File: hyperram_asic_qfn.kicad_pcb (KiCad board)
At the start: 4 copper layers, 59.5 x 60 mm, 45 parts, among them IC1 W25Q32JVSSIQ_TR, IC2 S27KL0641DABHI020, IC3 LP5907UVX-1.8_NOPB, IC4 LP5907UVX-3.3_NOPB, IC5 LP5907MFX-3.3_NOPB, IC6 MCP1824T-1802E_OT, J1 USB_B_Micro, J2 Conn_02x03_Counter_Clockwise, J3 1156915, J4 1156915, U1 CARAVEL, Y1 SG5032CAN_20.000000M-TJGA3

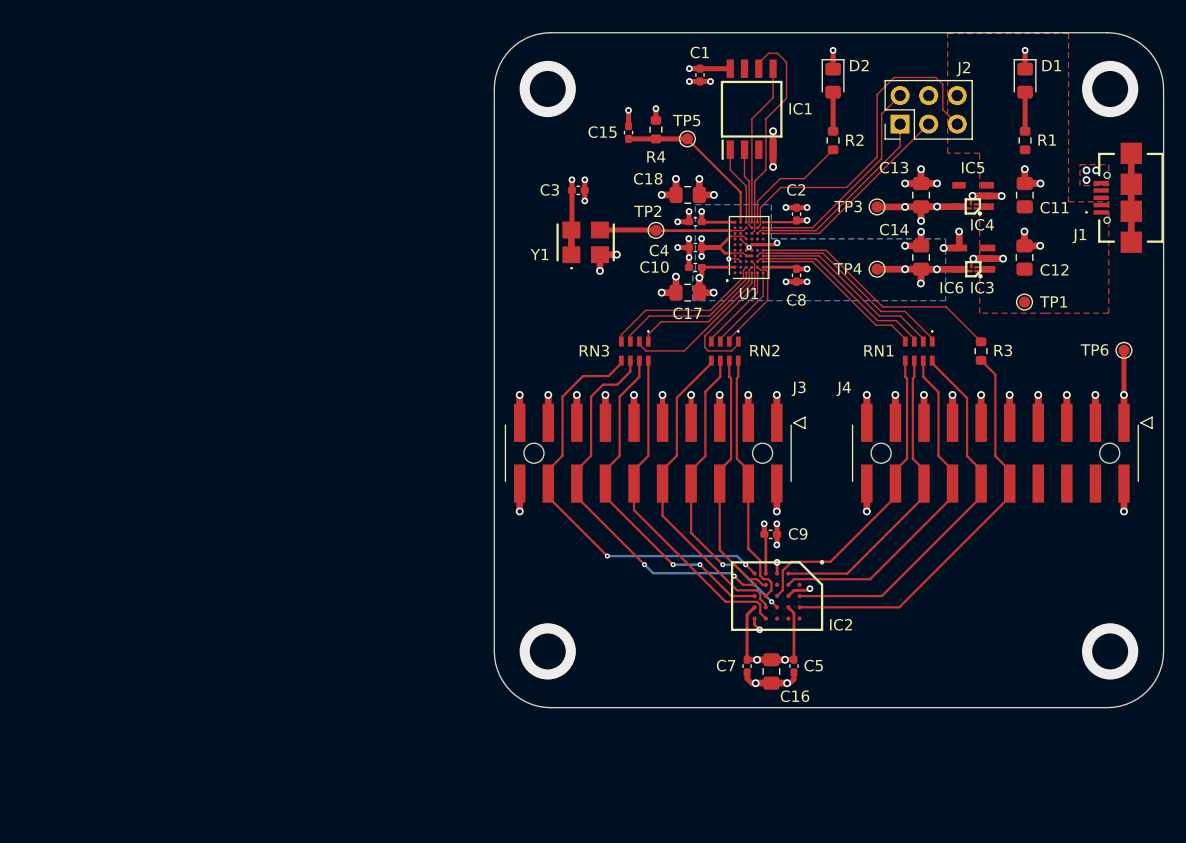
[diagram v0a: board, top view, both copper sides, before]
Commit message: First try on component placement and routing.
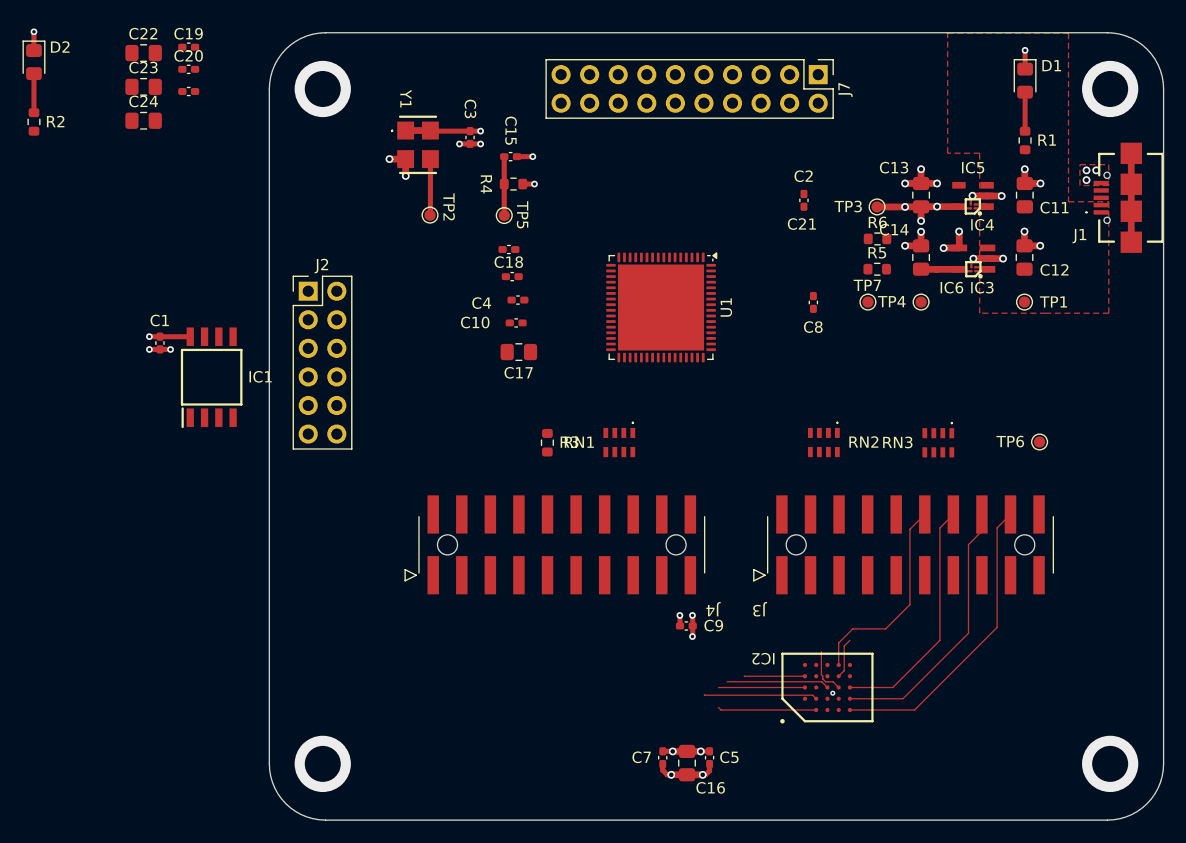
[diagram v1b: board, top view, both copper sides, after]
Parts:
- added C19: 100n, Capacitor_SMD:C_0402_1005Metric_Pad0.74x0.62mm_HandSolder, F.Cu at (115.3, 70.6)
- added C20: 100n, Capacitor_SMD:C_0402_1005Metric_Pad0.74x0.62mm_HandSolder, F.Cu at (115.3, 72.6)
- added C21: 100n, Capacitor_SMD:C_0402_1005Metric_Pad0.74x0.62mm_HandSolder, F.Cu at (115.3, 74.5)
- added C22: 22u 25v, Capacitor_SMD:C_0805_2012Metric_Pad1.18x1.45mm_HandSolder, F.Cu at (111.3, 71.1)
- added C23: 1u 16v, Capacitor_SMD:C_0805_2012Metric_Pad1.18x1.45mm_HandSolder, F.Cu at (111.3, 74.1)
- added C24: 22u 25v, Capacitor_SMD:C_0805_2012Metric_Pad1.18x1.45mm_HandSolder, F.Cu at (111.3, 77.1)
- added J7: Conn_02x10_Odd_Even, Connector_PinHeader_2.54mm:PinHeader_2x10_P2.54mm_Vertical, F.Cu at (171.3, 73.0)
- added R5: 0, Resistor_SMD:R_0603_1608Metric, F.Cu at (176.5, 90.3)
- added R6: NC, Resistor_SMD:R_0603_1608Metric, F.Cu at (176.6, 87.6)
- added TP7: TestPoint, TestPoint:TestPoint_Pad_D1.0mm, F.Cu at (175.7, 93.2)
- C10, C2, C4, C5, C6, C7, C8, C9: value 22n -> 100n
- C18: value 1u 16v -> 100n; footprint Capacitor_SMD:C_0805_2012Metric_Pad1.18x1.45mm_HandSolder -> Capacitor_SMD:C_0402_1005Metric_Pad0.74x0.62mm_HandSolder
- J2: value Conn_02x03_Counter_Clockwise -> Conn_02x06_Odd_Even; footprint Connector_PinHeader_2.54mm:PinHeader_2x03_P2.54mm_Vertical -> Connector_PinHeader_2.54mm:PinHeader_2x06_P2.54mm_Vertical
- R4: value 220 -> 2k2
- U1: value CARAVEL -> CARAVEL_QFN; footprint hyperram_asic_qfn:WLCSP-60_P0.5mm -> Package_DFN_QFN:QFN-64-1EP_9x9mm_P0.5mm_EP7.65x7.65mm
- moved D2 71.1 mm to (101.6, 71.9)
- moved R2 71.1 mm to (101.6, 77.2)
- moved J2 54.7 mm to (126.0, 92.3), turned to 0 degrees
- moved C1 53.6 mm to (112.8, 96.9)
- moved IC1 53.6 mm to (117.4, 99.9)
- moved R3 39.4 mm to (147.2, 105.7)
- moved J4 39.4 mm to (148.5, 114.8), turned to 180 degrees
- moved RN3 28.2 mm to (182.0, 105.8)
- moved RN1 27.8 mm to (153.6, 105.7)
- moved J3 24.7 mm to (179.5, 114.8), turned to 180 degrees
- moved TP2 20.1 mm to (136.8, 85.5), turned to -90 degrees
- moved TP5 17.6 mm to (143.4, 85.5), turned to -90 degrees
- moved Y1 17.2 mm to (135.7, 79.3), turned to -90 degrees
- moved C6 17.0 mm to (144.1, 91.0)
- moved C10 16.7 mm to (144.4, 95.1)
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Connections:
- C10 pad 1: +1V8 -> VCC
- C17 pad 1: +1V8 -> VCC
- C6 pad 1: +1V8 -> VCC
- C8 pad 1: +1V8 -> VCC
- J2 pad 1: /mgmt_spi_cs -> +3V3
- J2 pad 2: /mgmt_spi_di -> +3V3
- J2 pad 3: /mgmt_spi_clk -> GND
- J2 pad 6: +5V -> /mgmt_spi_di
- RN1 pad 1: /cvl_hr_csn -> /cvl_hr_rwds
- RN1 pad 2: /cvl_hr_clk -> /cvl_hr_clkn
- RN1 pad 3: /cvl_hr_clkn -> /cvl_hr_clk
- RN1 pad 4: /cvl_hr_rwds -> /cvl_hr_csn
- RN1 pad 5: /hr_rwds -> /hr_csn
- RN1 pad 6: /hr_clkn -> /hr_clk
- RN1 pad 7: /hr_clk -> /hr_clkn
- RN1 pad 8: /hr_csn -> /hr_rwds
- RN2 pad 1: /cvl_hr_dq0 -> /cvl_hr_dq3
- RN2 pad 2: /cvl_hr_dq1 -> /cvl_hr_dq2
- RN2 pad 3: /cvl_hr_dq2 -> /cvl_hr_dq1
- RN2 pad 4: /cvl_hr_dq3 -> /cvl_hr_dq0
- RN2 pad 5: /hr_dq3 -> /hr_dq0
- RN2 pad 6: /hr_dq2 -> /hr_dq1
- RN2 pad 7: /hr_dq1 -> /hr_dq2
- RN2 pad 8: /hr_dq0 -> /hr_dq3
- RN3 pad 1: /cvl_hr_dq4 -> /cvl_hr_dq7
- RN3 pad 2: /cvl_hr_dq5 -> /cvl_hr_dq6
- RN3 pad 3: /cvl_hr_dq6 -> /cvl_hr_dq5
- RN3 pad 4: /cvl_hr_dq7 -> /cvl_hr_dq4
- RN3 pad 5: /hr_dq7 -> /hr_dq4
- RN3 pad 6: /hr_dq6 -> /hr_dq5
- RN3 pad 7: /hr_dq5 -> /hr_dq6
- RN3 pad 8: /hr_dq4 -> /hr_dq7
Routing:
- net GND: track 132.3 -> 40.9 mm, vias 80 -> 35
- net /hr_rstn: track 35.9 -> 5.40 mm
- net /mgmt_spi_do: track 30.4 -> 0.00 mm
- net +3V3: track 55.4 -> 26.1 mm, vias 14 -> 9
- net /hr_dq2: track 26.8 -> 0.00 mm, vias 2 -> 0
- net /hr_csn: track 33.7 -> 7.68 mm
- net /hr_dq3: track 28.6 -> 3.61 mm
- net /cvl_hr_rstn: track 22.7 -> 0.00 mm
- net /hr_dq1: track 22.7 -> 0.00 mm
- net /hr_clk: track 31.0 -> 10.1 mm
- net /flash_clk: track 20.1 -> 0.00 mm
- net +1V8: track 24.2 -> 4.55 mm, vias 7 -> 0
- net /mgmt_spi_di: track 19.4 -> 0.00 mm
- net /cvl_hr_csn: track 19.0 -> 0.00 mm
- net /mgmt_spi_clk: track 18.7 -> 0.00 mm
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- removed copper zone on B.Cu, net +1V8
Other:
- board size 59.5 x 60 mm -> 79.5 x 70 mm
